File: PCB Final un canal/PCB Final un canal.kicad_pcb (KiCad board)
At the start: 2 copper layers, 55.2 x 50 mm, 32 parts, among them J1 Conn_01x02, J2 Conn_01x03, J3 Conn_01x02, U1 LM324, U2 AD620, U3 LM324

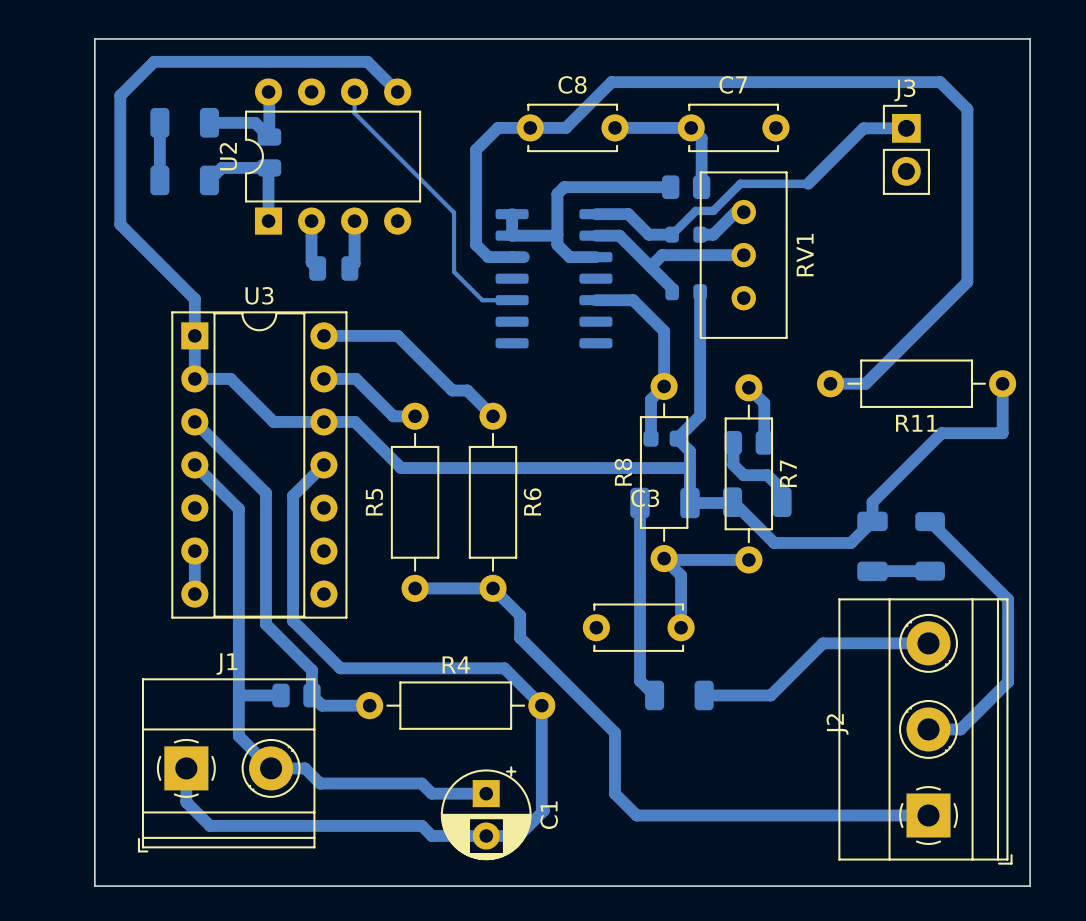
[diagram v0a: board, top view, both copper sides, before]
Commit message: Agrego la PCB con smd terminada de routear
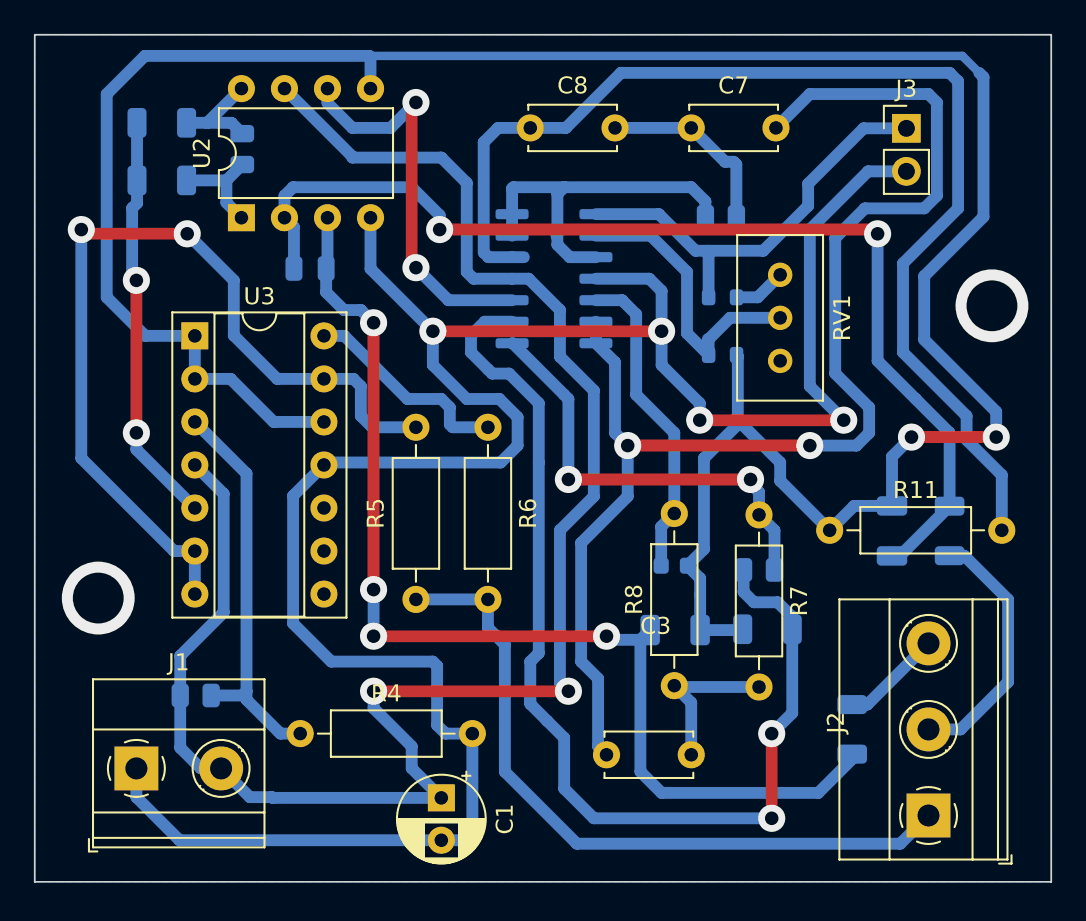
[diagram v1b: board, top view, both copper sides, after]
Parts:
- moved R11 13.4 mm to (69.7, 48.2), turned to 0 degrees
- moved R10 10.4 mm to (71.0, 60.0), turned to -90 degrees
- moved C2 7.52 mm to (60.5, 50.3)
- moved C3 7.52 mm to (56.5, 61.5)
- moved C6 7.52 mm to (60.5, 54.1)
- moved R15 7.52 mm to (66.0, 54.1)
- moved R17 7.52 mm to (65.5, 50.6)
- moved R7 7.52 mm to (65.5, 47.3)
- moved R8 7.52 mm to (60.5, 57.4)
- moved R3 5.95 mm to (32.2, 58.0)
- moved R4 4.42 mm to (38.4, 60.2)
- moved RV1 4.28 mm to (66.8, 38.2)
- moved R16 4.28 mm to (63.4, 34.5)
- moved R14 4.28 mm to (63.4, 37.9)
- moved J1 2.95 mm to (28.8, 62.3)
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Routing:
- net -V: track 57.5 -> 138.2 mm, vias 0 -> 4
- net Net-(C3-Pad1): track 0.00 -> 78.1 mm, vias 0 -> 2
- net +V: track 35.7 -> 103.7 mm, vias 0 -> 2
- net OutNEg: track 6.35 -> 64.1 mm, vias 0 -> 2
- net Net-(R15-Pad1): track 5.51 -> 62.9 mm, vias 0 -> 2
- net OutPosit: track 14.6 -> 65.0 mm, vias 0 -> 4
- net GND: track 106.9 -> 151.9 mm, vias 0 -> 2
- net Net-(R5-Pad2): track 8.83 -> 52.5 mm, vias 0 -> 2
- net OUT2: track 3.63 -> 26.1 mm, vias 0 -> 2
- net Net-(R1-Pad2): track 3.68 -> 24.4 mm, vias 0 -> 2
- net ElecPosit: track 14.5 -> 6.00 mm
- net Net-(C8-Pad1): track 60.8 -> 69.2 mm
- net Net-(C2-Pad2): track 11.4 -> 18.8 mm
- net OUT1: track 17.2 -> 23.7 mm, vias 0 -> 2
- net Net-(R14-Pad2): track 11.6 -> 17.4 mm
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- added copper zone on B.Cu, net GND
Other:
- board size 55.2 x 50 mm -> 60 x 50 mm
